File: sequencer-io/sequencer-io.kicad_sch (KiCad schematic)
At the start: 97 parts, among them SW1 SW_Push, SW10 SW_Push, SW11 SW_Push, SW12 SW_Push, SW13 SW_Push, SW14 SW_Push, SW15 SW_Push, SW16 SW_Push, SW17 SW_Push, SW18 SW_Push, SW19 SW_Push, SW2 SW_Push, SW20 SW_Push, SW21 SW_Push, SW22 SW_Push, SW23 SW_Push, SW24 RotaryEncoder, SW3 SW_Push, SW4 SW_Push, SW5 SW_Push, SW6 SW_Push, SW7 SW_Push, SW8 SW_Push, SW9 SW_Push, U2 74HC595, U20 SC0915

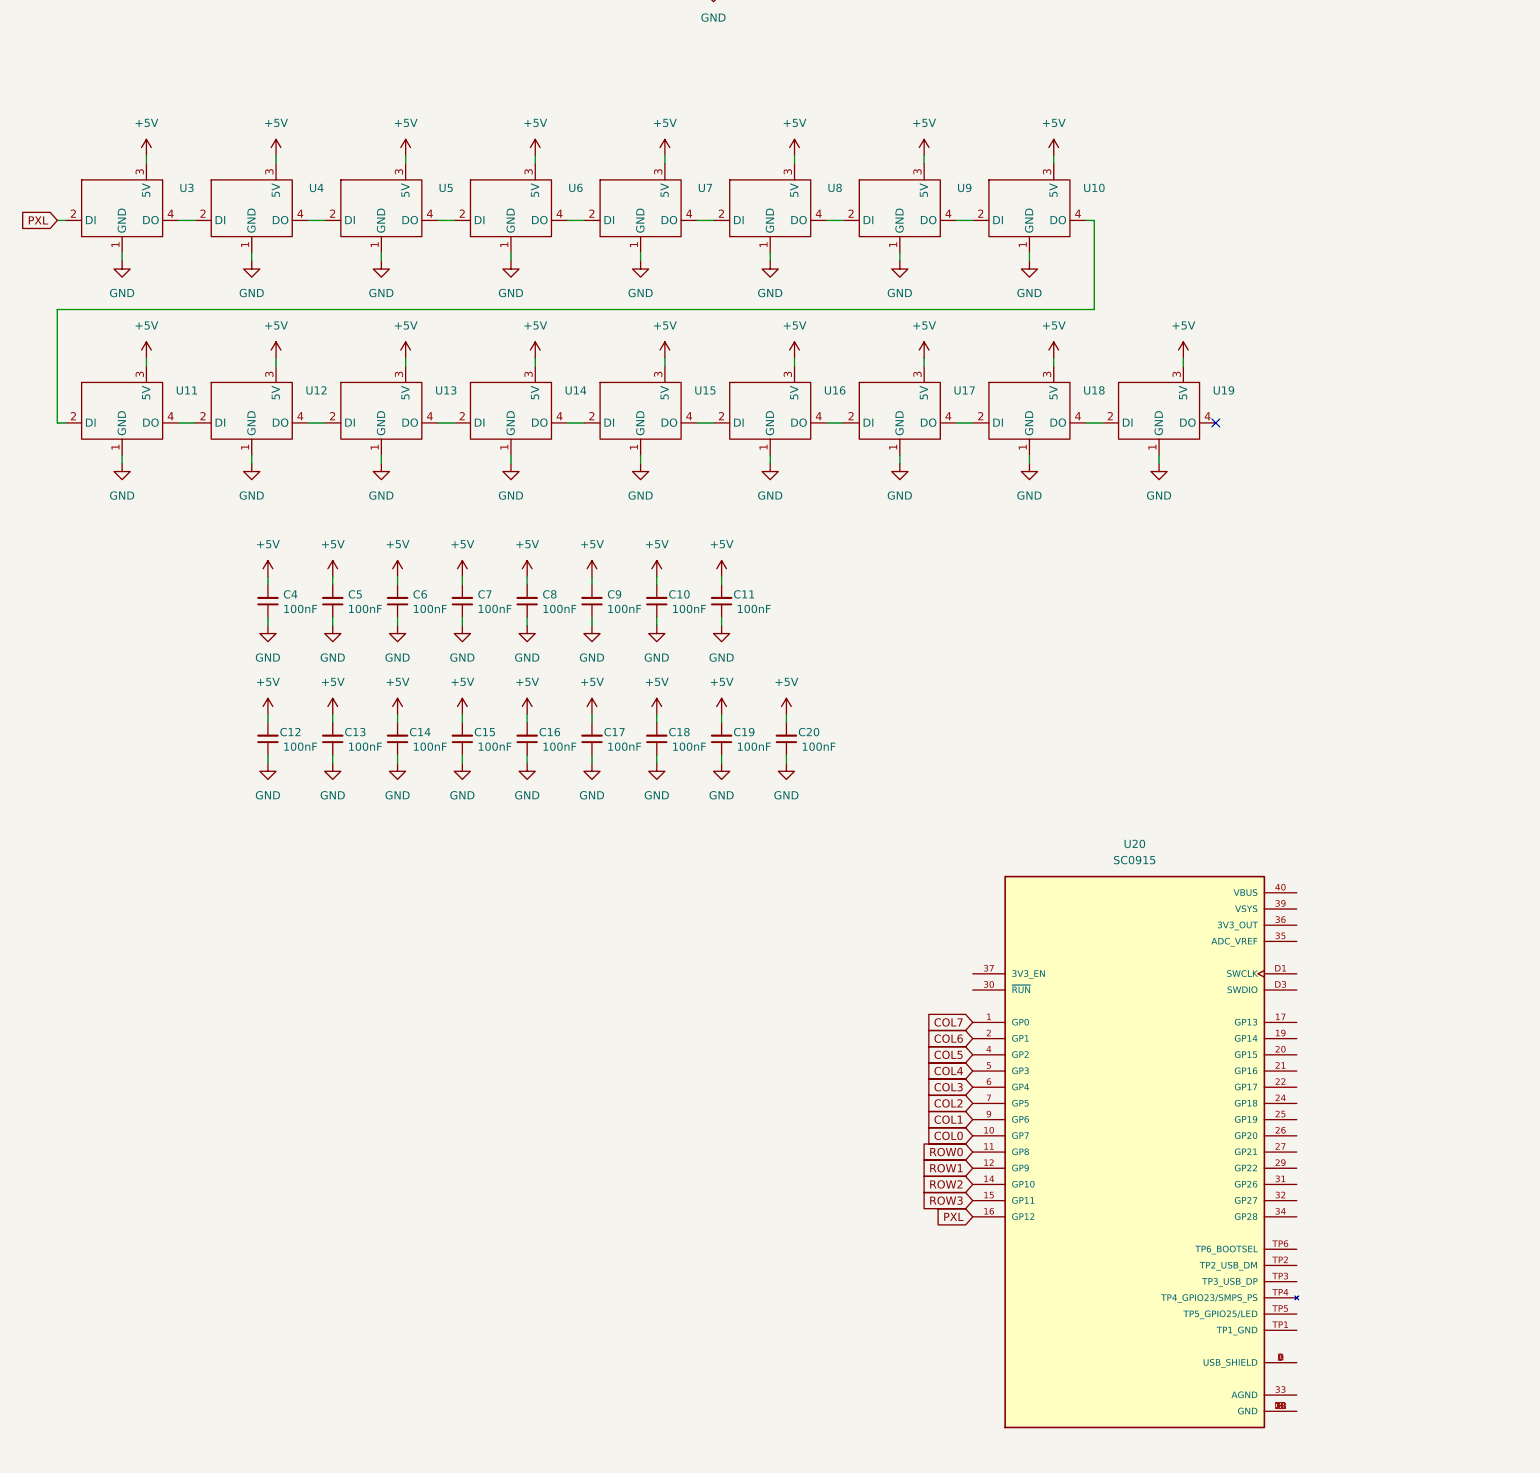
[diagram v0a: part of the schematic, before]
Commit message: Edited PCB
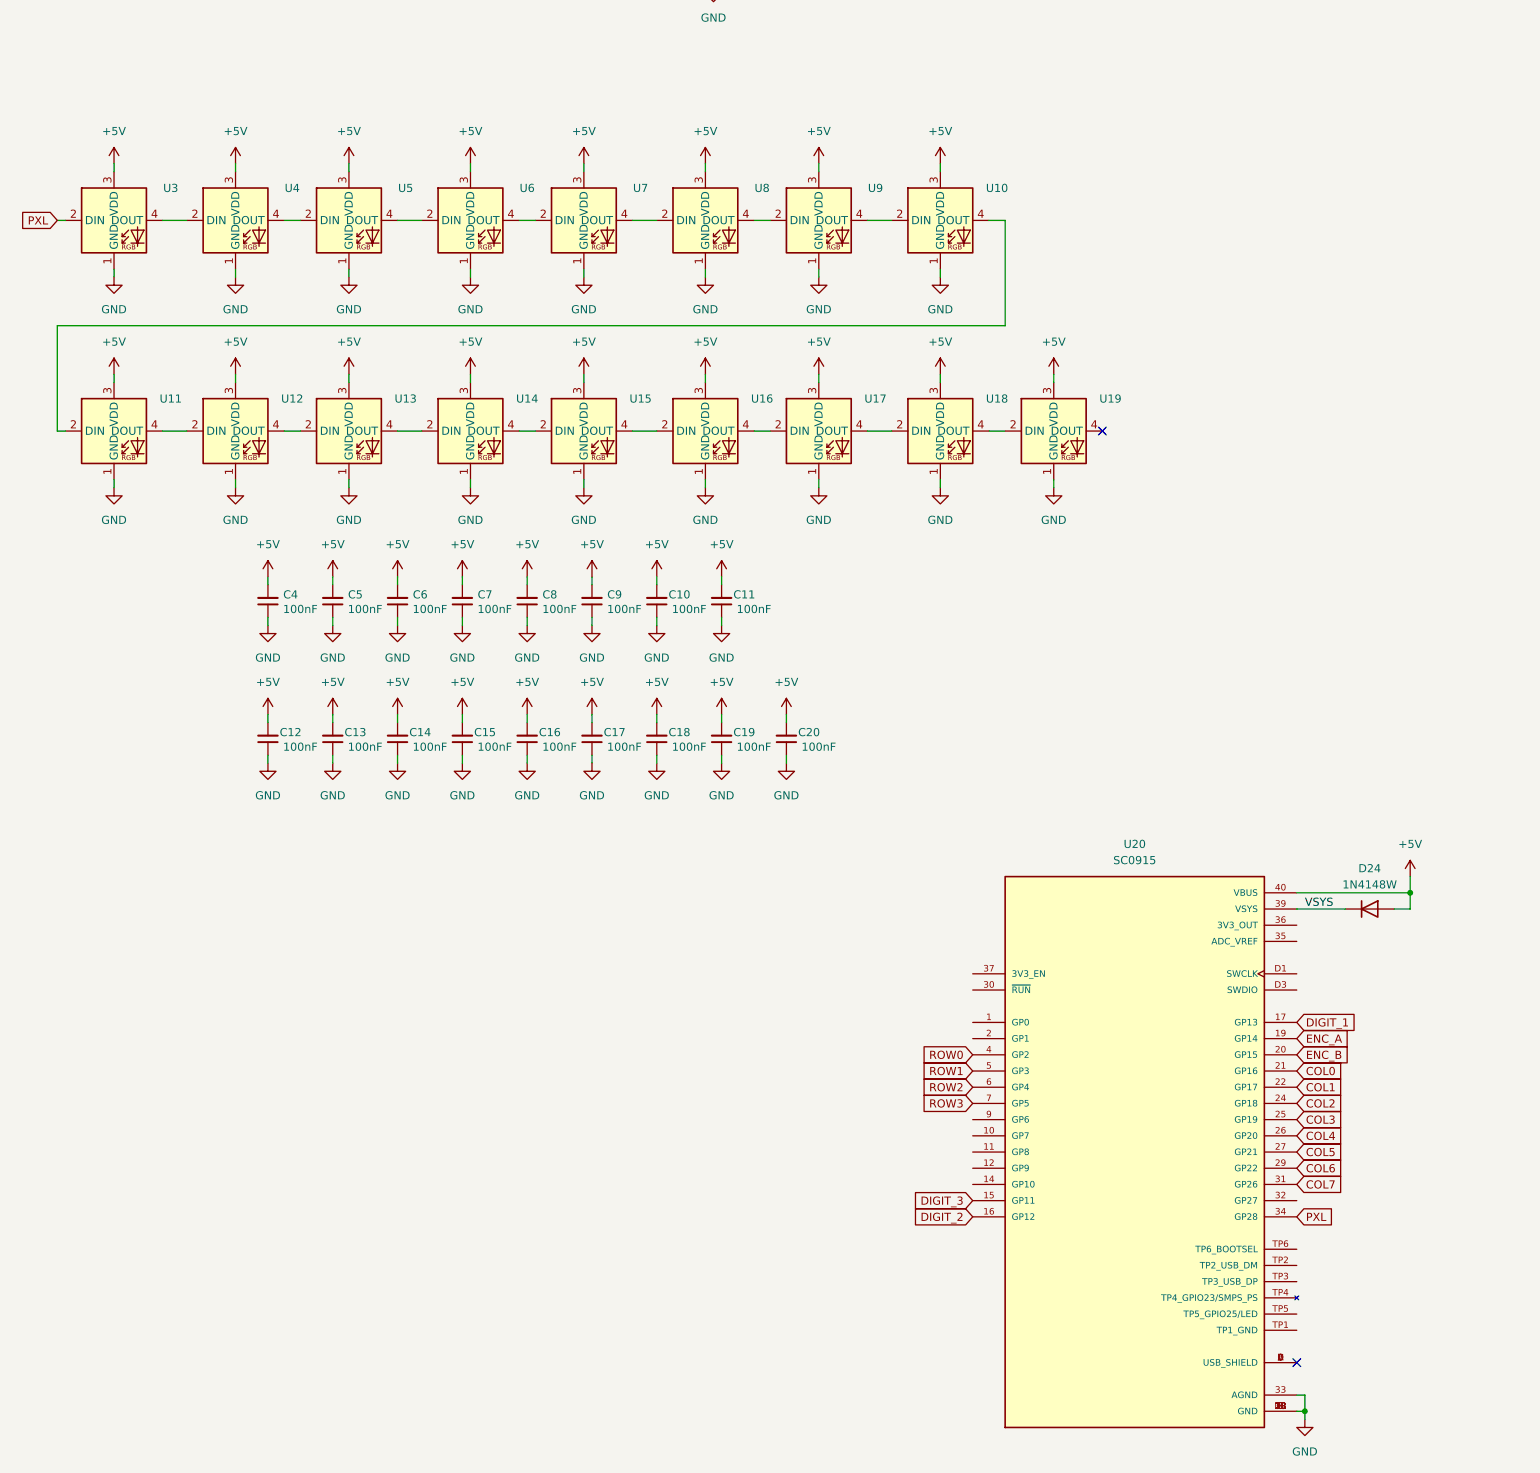
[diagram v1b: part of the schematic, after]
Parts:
- added D24: 1N4148W, Diode_SMD:D_SOD-323_HandSoldering, symbol Diode:1N4148W
- U20: footprint SC0915:MODULE_SC0915 -> SC0915:SC0915
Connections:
- net +5V: now also U20.40 (VBUS), D24.2 (A)
- net COL0: now also U20.21 (GP16); no longer U20.10 (GP7)
- net COL1: now also U20.22 (GP17); no longer U20.9 (GP6)
- net COL2: now also U20.24 (GP18); no longer U20.7 (GP5)
- net COL3: now also U20.25 (GP19); no longer U20.6 (GP4)
- net COL4: now also U20.26 (GP20); no longer U20.5 (GP3)
- net COL5: now also U20.27 (GP21); no longer U20.4 (GP2)
- net COL6: now also U20.29 (GP22); no longer U20.2 (GP1)
- net COL7: now also U20.31 (GP26); no longer U20.1 (GP0)
- net DIGIT_1: now also U20.17 (GP13)
- net DIGIT_2: now also U20.16 (GP12)
- net DIGIT_3: now also U20.15 (GP11)
- net ENC_A: now also U20.19 (GP14)
- net ENC_B: now also U20.20 (GP15)
- net GND: now also U20.13 (GND), U20.18 (GND), U20.23 (GND), U20.28 (GND), U20.3 (GND), U20.33 (AGND), U20.38 (GND), U20.8 (GND), U20.D2 (GND)
- net PXL: now also U20.34 (GP28); no longer U20.16 (GP12)
- net ROW0: now also U20.4 (GP2); no longer U20.11 (GP8)
- net ROW1: now also U20.5 (GP3); no longer U20.12 (GP9)
- net ROW2: now also U20.6 (GP4); no longer U20.14 (GP10)
- net ROW3: now also U20.7 (GP5); no longer U20.15 (GP11)
- net VSYS: now reaches U20.39 (VSYS)
- net VSYS: now also D24.1 (K)
- no-connect marks 1 -> 2
